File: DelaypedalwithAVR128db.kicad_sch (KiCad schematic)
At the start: 23 parts, among them J1 NJ2FD-V, J2 NJ2FD-V, K1 Relay_SPDT, U1 TLV9002, U2 TLV9002

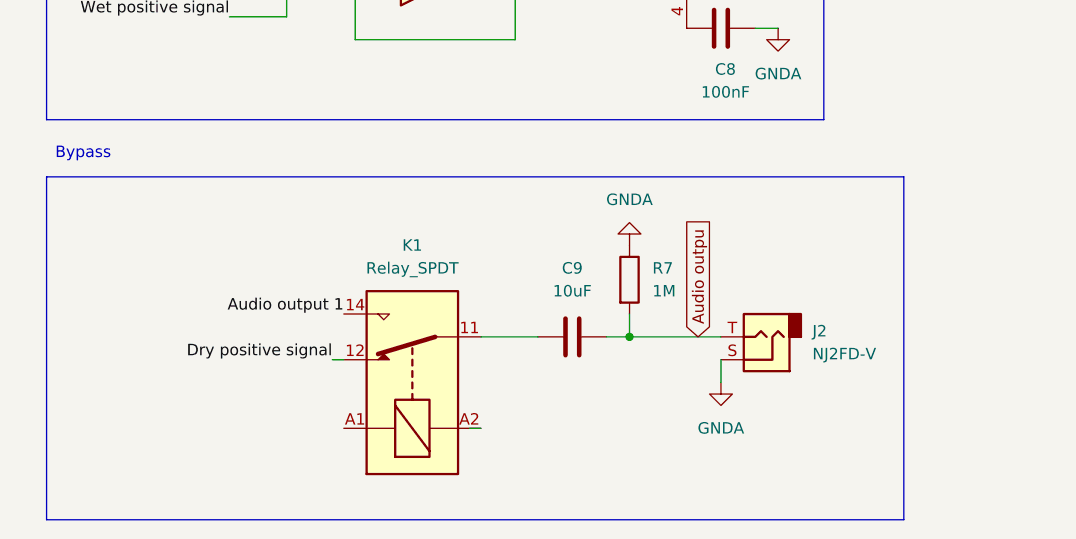
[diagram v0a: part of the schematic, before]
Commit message: Bypass finished???
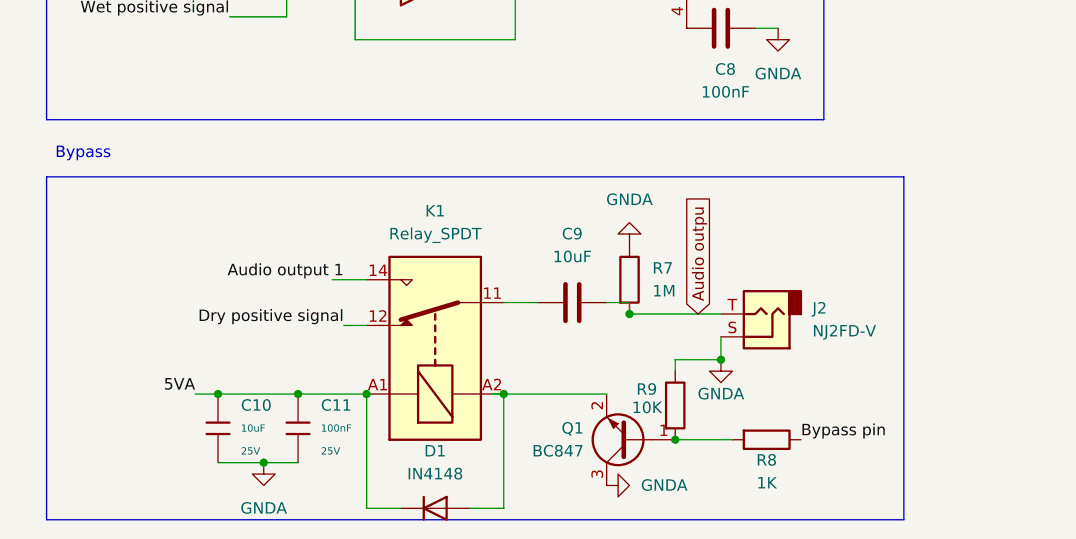
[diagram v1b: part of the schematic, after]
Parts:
- added C10: 10uF, PCM_JLCPCB:C_1206, symbol PCM_JLCPCB-Capacitors:1206,10uF
- added C11: 100nF, PCM_JLCPCB:C_1206, symbol PCM_JLCPCB-Capacitors:1206,100nF
- added D1: IN4148, symbol Device:D
- added Q1: BC847, Package_TO_SOT_SMD:SOT-23, symbol Transistor_BJT:BC847
- added R8: 1K, symbol Device:R
- added R9: 10K, symbol Device:R
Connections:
- net 5VA: now also K1.A1, C10.1, C11.1, D1.1 (K)
- net GNDA: now also C10.2, C11.2, Q1.3 (C), R9.1
- net at K1.A2: now also D1.2 (A), Q1.2 (E)
- new net: Q1.1 (B), R8.2, R9.2
- new net Bypass pin: R8.1
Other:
- moved on the sheet: C9, J2, K1
